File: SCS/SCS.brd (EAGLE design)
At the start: 122.8 x 81 mm, 20 parts, among them IC1 74HC165D

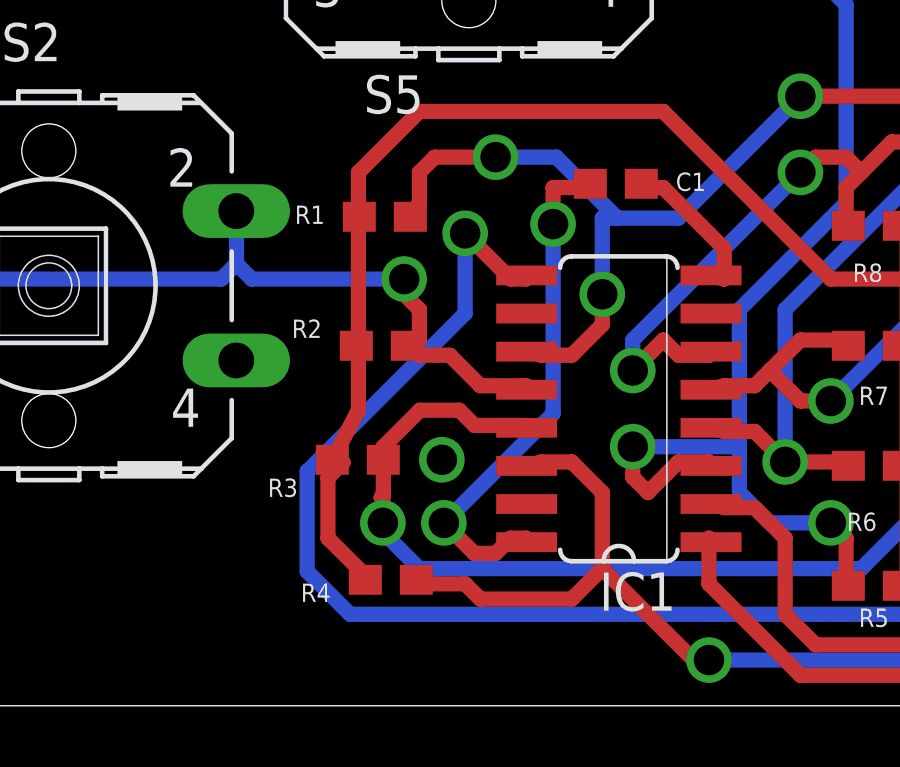
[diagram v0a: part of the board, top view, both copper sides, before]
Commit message: Adjustments to PCB Signed-off-by: goslo <digit99@mailinator.com>
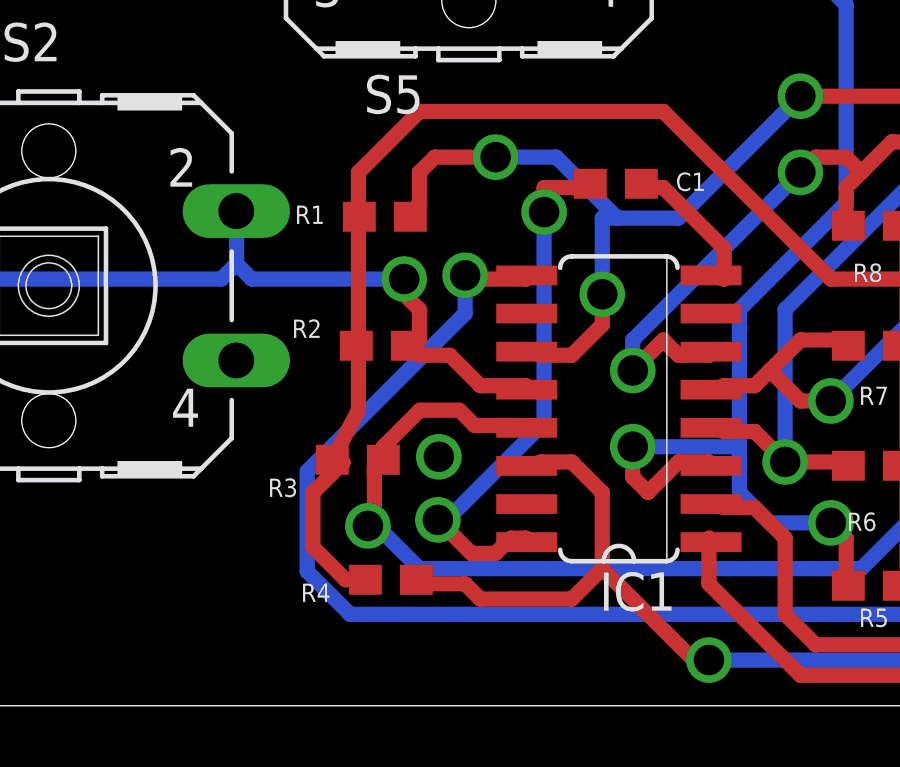
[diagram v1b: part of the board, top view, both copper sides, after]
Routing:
- net N$4: track 57.0 -> 55.0 mm
- net VCC: track 59.1 -> 60.0 mm
- net N$12: track 17.5 -> 18.1 mm
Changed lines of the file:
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@@
 <contactref element="ENC1" pad="D"/>
 <contactref element="J1" pad="1"/>
-<polygon width="0.0762" layer="1">
+<polygon width="0.5" layer="1">
 <vertex x="-2" y="86"/>
 <vertex x="130" y="86"/>
@@
 <vertex x="-2" y="-6"/>
 </polygon>
-<polygon width="0.0762" layer="16">
+<polygon width="0.5" layer="16">
 <vertex x="-2" y="86"/>
 <vertex x="130" y="86"/>
@@
 <vertex x="-2" y="-6"/>
 </polygon>
-<via x="23.1" y="8.2" extent="1-16" drill="1.016"/>
+<via x="23" y="8.3" extent="1-16" drill="1.016"/>
 </signal>
 <signal name="B-">
@@
 <contactref element="J8/9" pad="3"/>
 <contactref element="J8/9" pad="4"/>
-<wire x1="19.304" y1="5.588" x2="20.32" y2="4.572" width="0.508" layer="1"/>
-<wire x1="19.304" y1="7.604" x2="19.304" y2="5.588" width="0.508" layer="1"/>
-<wire x1="19.807428125" y1="8.107428125" x2="19.304" y2="7.604" width="0.508" layer="1"/>
-<wire x1="20.32" y1="4.572" x2="20.55" y2="4.2" width="0.508" layer="1"/>
+<wire x1="20.55" y1="4.2" x2="19.892" y2="4.2" width="0.508" layer="1"/>
+<wire x1="19.892" y1="4.2" x2="18.804" y2="5.288" width="0.508" layer="1"/>
+<wire x1="18.804" y1="7.104" x2="18.804" y2="5.288" width="0.508" layer="1"/>
+<wire x1="19.807428125" y1="8.107428125" x2="18.804" y2="7.104" width="0.508" layer="1"/>
 <wire x1="19.807428125" y1="8.107428125" x2="19.45" y2="8.2" width="0.508" layer="1"/>
 <wire x1="20.32" y1="9.84921875" x2="20.32" y2="11.684" width="0.508" layer="1"/>
@@
 <wire x1="25.9266" y1="9.265" x2="25.8476" y2="9.344" width="0.508" layer="1"/>
 <wire x1="25.8476" y1="9.344" x2="24.192" y2="9.344" width="0.508" layer="1"/>
-<wire x1="21.136" y1="7.004" x2="21.077378125" y2="6.945378125" width="0.508" layer="1"/>
-<wire x1="21.136" y1="6.096" x2="21.136" y2="7.004" width="0.508" layer="1"/>
-<wire x1="21.136" y1="6.096" x2="21.136" y2="5.788" width="0.508" layer="16"/>
-<wire x1="22.352" y1="4.572" x2="21.136" y2="5.788" width="0.508" layer="16"/>
+<wire x1="21.15" y1="8.2" x2="20.85" y2="7.9" width="0.508" layer="1"/>
+<wire x1="20.85" y1="7.9" x2="20.85" y2="6.21" width="0.508" layer="1"/>
+<wire x1="20.636" y1="5.996" x2="20.85" y2="6.21" width="0.508" layer="1"/>
+<wire x1="20.636" y1="5.996" x2="20.928" y2="5.996" width="0.508" layer="16"/>
+<wire x1="22.352" y1="4.572" x2="20.928" y2="5.996" width="0.508" layer="16"/>
 <wire x1="37.084" y1="4.572" x2="22.352" y2="4.572" width="0.508" layer="16"/>
 <wire x1="42.164" y1="9.652" x2="37.084" y2="4.572" width="0.508" layer="16"/>
@@
 <wire x1="67.056" y1="23.368" x2="65.024" y2="21.336" width="0.508" layer="16"/>
 <wire x1="68.072" y1="25.4" x2="68.072" y2="24.384" width="0.508" layer="16"/>
-<wire x1="21.15" y1="7.048259375" x2="21.15" y2="8.2" width="0.508" layer="1"/>
-<wire x1="21.15" y1="7.048259375" x2="21.077378125" y2="6.945378125" width="0.508" layer="1"/>
 <wire x1="68.072" y1="25.4" x2="67.7516" y2="25.5108" width="0.508" layer="16"/>
 <wire x1="78.74" y1="25.4" x2="79.756" y2="25.4" width="0.508" layer="16"/>
@@
 <wire x1="67.056" y1="23.368" x2="69.088" y2="21.336" width="0.508" layer="16"/>
 <wire x1="79.756" y1="25.4" x2="80.2484" y2="25.5108" width="0.508" layer="16"/>
-<via x="21.136" y="6.096" extent="1-16" drill="1.016"/>
+<via x="20.636" y="5.996" extent="1-16" drill="1.016"/>
 </signal>
 <signal name="N$3">
@@
 <contactref element="IC1" pad="9"/>
 <contactref element="J8/9" pad="5"/>
-<wire x1="25.4" y1="14.224" x2="25.908" y2="14.224" width="0.508" layer="1"/>
-<wire x1="23.876" y1="15.748" x2="25.4" y2="14.224" width="0.508" layer="1"/>
-<wire x1="23.876" y1="13.076" x2="23.876" y2="15.748" width="0.508" layer="16"/>
+<wire x1="24" y1="14.224" x2="25.908" y2="14.224" width="0.508" layer="1"/>
+<wire x1="23.876" y1="14.348" x2="24" y2="14.224" width="0.508" layer="1"/>
+<wire x1="23.876" y1="13.076" x2="23.876" y2="14.348" width="0.508" layer="16"/>
 <wire x1="18.612" y1="7.812" x2="23.876" y2="13.076" width="0.508" layer="16"/>
 <wire x1="18.612" y1="4.48" x2="18.612" y2="7.812" width="0.508" layer="16"/>
@@
 <wire x1="25.908" y1="14.224" x2="25.9266" y2="14.345" width="0.508" layer="1"/>
 <wire x1="47.244" y1="10.668" x2="47.437" y2="10.71" width="0.508" layer="16"/>
-<via x="23.876" y="15.748" extent="1-16" drill="1.016"/>
+<via x="23.876" y="14.348" extent="1-16" drill="1.016"/>
 </signal>
 <signal name="SC">
@@
 <contactref element="IC1" pad="16"/>
 <contactref element="C1" pad="1"/>
-<wire x1="26.808" y1="17.272" x2="27.94" y2="17.272" width="0.508" layer="1"/>
-<wire x1="26.808" y1="16.056" x2="26.808" y2="17.272" width="0.508" layer="1"/>
-<wire x1="26.808" y1="16.056" x2="26.808" y2="9.736" width="0.508" layer="16"/>
-<wire x1="23.168" y1="6.096" x2="26.808" y2="9.736" width="0.508" layer="16"/>
-<wire x1="24.184" y1="5.08" x2="23.168" y2="6.096" width="0.508" layer="1"/>
-<wire x1="24.892" y1="5.08" x2="24.184" y2="5.08" width="0.508" layer="1"/>
+<wire x1="26.508" y1="17.272" x2="27.94" y2="17.272" width="0.508" layer="1"/>
+<wire x1="26.508" y1="16.456" x2="26.508" y2="17.272" width="0.508" layer="1"/>
+<wire x1="26.508" y1="16.456" x2="26.508" y2="9.436" width="0.508" layer="16"/>
+<wire x1="26.508" y1="9.436" x2="23.268" y2="6.196" width="0.508" layer="16"/>
+<wire x1="22.968" y1="6.196" x2="23.268" y2="6.196" width="0.508" layer="16"/>
+<wire x1="24.084" y1="5.08" x2="22.968" y2="6.196" width="0.508" layer="1"/>
+<wire x1="24.892" y1="5.08" x2="24.084" y2="5.08" width="0.508" layer="1"/>
 <wire x1="25.4" y1="5.588" x2="24.892" y2="5.08" width="0.508" layer="1"/>
 <wire x1="25.908" y1="5.588" x2="25.4" y2="5.588" width="0.508" layer="1"/>
 <wire x1="27.94" y1="17.272" x2="28.05" y2="17.4" width="0.508" layer="1"/>
 <wire x1="25.908" y1="5.588" x2="25.9266" y2="5.455" width="0.508" layer="1"/>
-<via x="26.808" y="16.056" extent="1-16" drill="1.016"/>
-<via x="23.168" y="6.096" extent="1-16" drill="1.016"/>
+<via x="26.508" y="16.456" extent="1-16" drill="1.016"/>
+<via x="22.968" y="6.196" extent="1-16" drill="1.016"/>
 </signal>
 <signal name="N$13">
